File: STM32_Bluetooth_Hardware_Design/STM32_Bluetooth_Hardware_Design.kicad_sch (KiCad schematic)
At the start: 41 parts, among them J1 Conn_Coaxial, J2 Conn_ARM_SWD_TagConnect_TC2030, J3 USB_C_Receptacle_USB2.0_16P, J4 Conn_01x04, SW1 SW_Push, U1 STM32WB55CEUx, U2 USBLC6-2SC6, U3 MIC5365-3.3YD5, X1 32kHz768, X2 32MHz

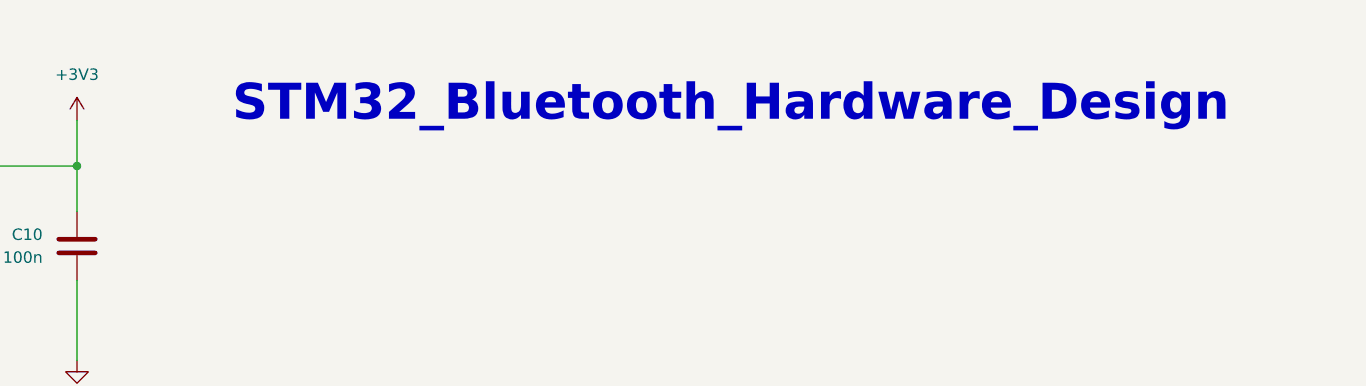
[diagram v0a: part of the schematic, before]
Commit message: STM32 UART
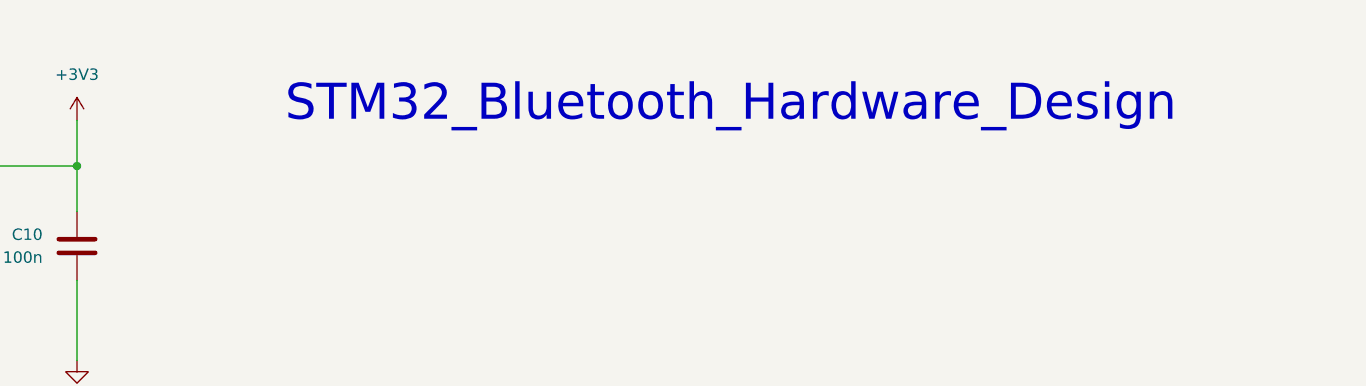
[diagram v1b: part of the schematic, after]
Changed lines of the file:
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@@
 			(font
 				(size 4 4)
-				(thickness 0.4)
-				(bold yes)
-				(color 53 20 255 1)
+				(thickness 0.5)
+				(color 0 0 0 1)
 			)
 		)
